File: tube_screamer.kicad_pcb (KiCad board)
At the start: 2 copper layers, 35 parts, among them Q1 BC817, U1 TL072

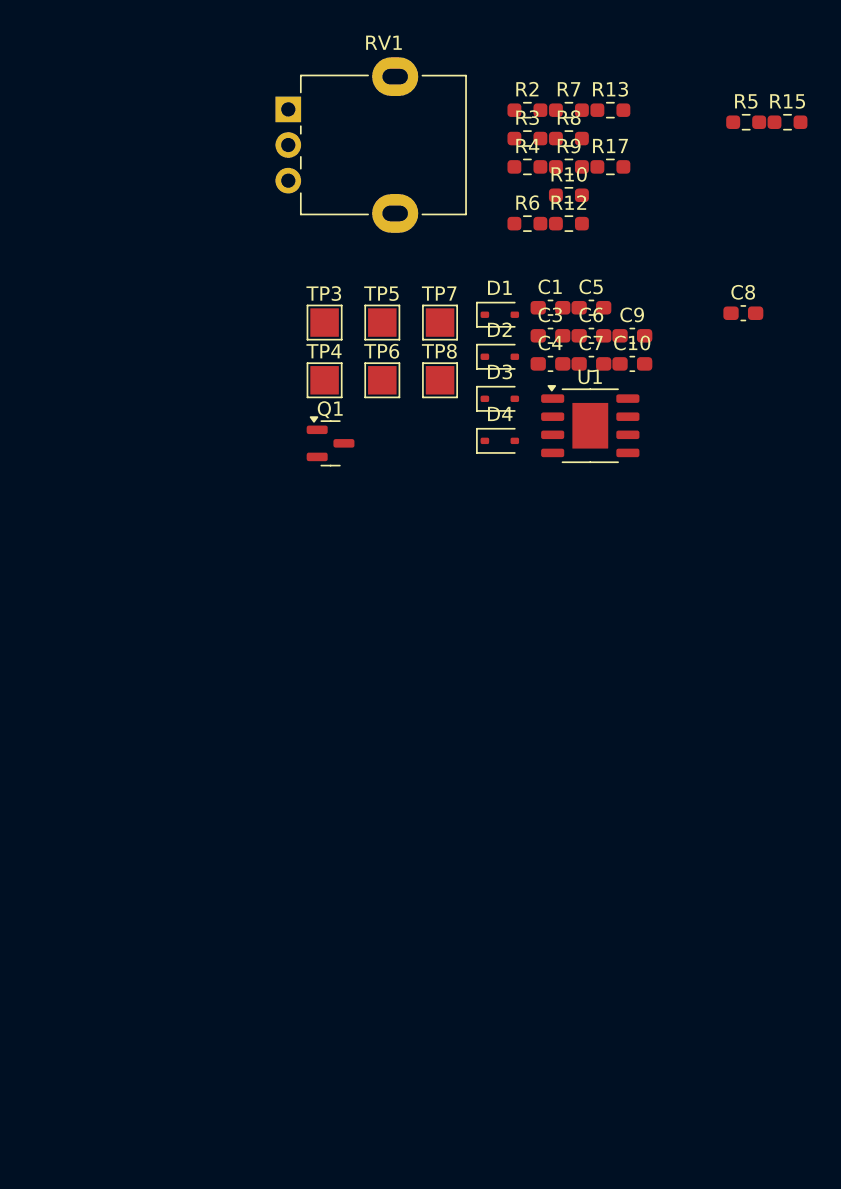
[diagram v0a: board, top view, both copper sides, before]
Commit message: PCB layout.
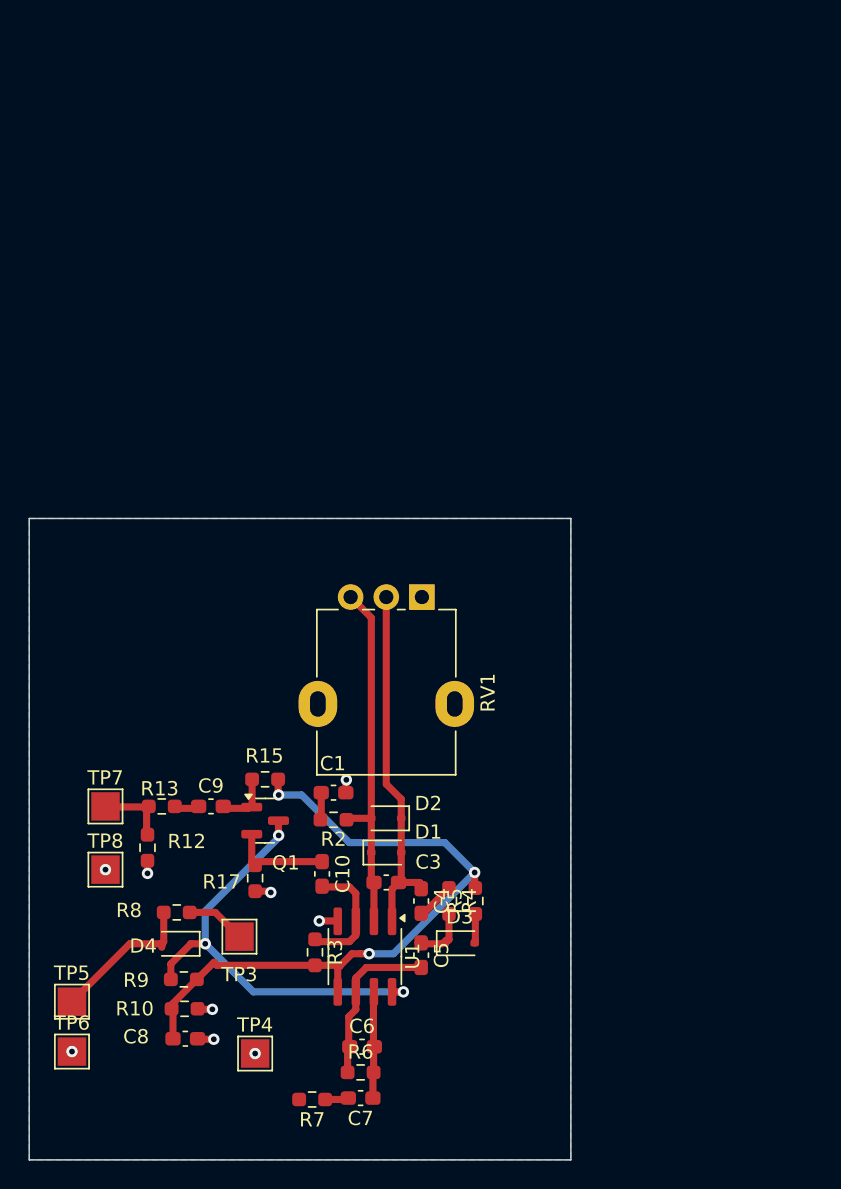
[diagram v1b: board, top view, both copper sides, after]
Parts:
- U1: footprint Package_SO:SOIC-8-1EP_3.9x4.9mm_P1.27mm_EP2.514x3.2mm -> Package_SO:SOIC-8_3.9x4.9mm_P1.27mm
- moved R7 71.7 mm to (119.8, 140.8), turned to 180 degrees
- moved C8 64.2 mm to (111.0, 136.5), turned to 180 degrees
- moved R10 63.1 mm to (110.9, 134.4)
- moved R9 63.1 mm to (110.8, 132.3)
- moved R8 60.9 mm to (110.3, 127.6), turned to 180 degrees
- moved R6 60.7 mm to (123.2, 138.9)
- moved R3 59.0 mm to (120.0, 130.4), turned to -90 degrees
- moved R15 58.9 mm to (116.5, 118.3), turned to 180 degrees
- moved R13 58.1 mm to (109.3, 120.2), turned to 180 degrees
- moved R5 57.8 mm to (131.3, 126.8), turned to 90 degrees
- moved R17 55.8 mm to (115.8, 125.2), turned to -90 degrees
- moved C7 54.0 mm to (123.2, 140.7), turned to 180 degrees
- moved R12 52.8 mm to (108.3, 123.1), turned to -90 degrees
- moved C6 52.4 mm to (123.3, 137.1)
- moved TP5 52.4 mm to (103.0, 133.9)
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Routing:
- net 4V5: track 0.00 -> 47.8 mm, vias 0 -> 3
- net 9V: track 0.00 -> 31.0 mm, vias 0 -> 3
- net Net-(D1-A): track 0.00 -> 25.3 mm
- net Net-(D1-K): track 0.00 -> 25.2 mm
- net Net-(U1B--): track 0.00 -> 11.5 mm
- net Net-(D4-A): track 0.00 -> 10.5 mm
- net Net-(U1A-+): track 0.00 -> 8.63 mm
- net Net-(C6-Pad2): track 0.00 -> 7.53 mm
- net Net-(Q1-E): track 0.00 -> 7.08 mm
- net 0: track 0.00 -> 6.37 mm, vias 0 -> 9
- net Net-(R12-Pad1): track 0.00 -> 4.92 mm
- net Net-(R8-Pad1): track 0.00 -> 4.19 mm
- net Net-(D3-K): track 0.00 -> 4.14 mm
- net Net-(Q1-B): track 0.00 -> 3.90 mm
- net Net-(C4-Pad2): track 0.00 -> 2.64 mm
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- added copper zone on B.Cu, net 0
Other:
- board outline added: 38 x 45 mm
